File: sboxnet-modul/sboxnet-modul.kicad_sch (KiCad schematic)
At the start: 33 parts, among them J2 Conn_02x03_Odd_Even, J4 8P8C, J5 8P8C, J6 sboxnet-buchse_2x17, SW1 SW_Push, U1 MCP1703A-3302_SOT223, U2 MCP1703A-5002_SOT223, U3 SN65HVD230, U4 ATxmega128A4U-AU, Y1 16MHz

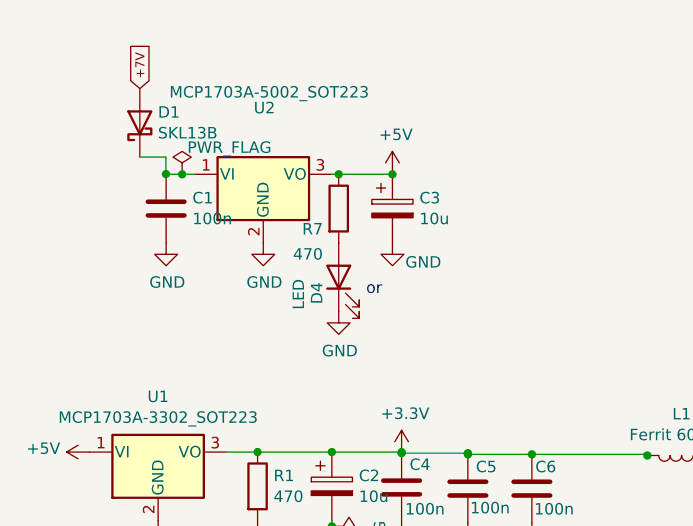
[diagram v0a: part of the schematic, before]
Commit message: sboxnet modul V6
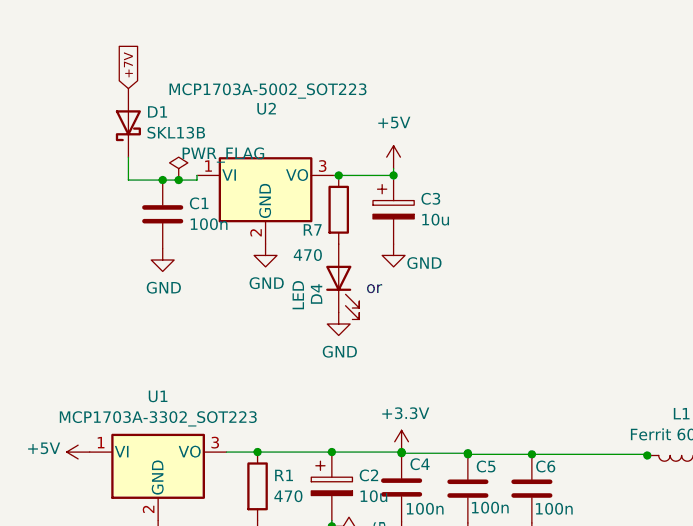
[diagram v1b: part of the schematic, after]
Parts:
- C3: footprint Capacitor_SMD:C_1206_3216Metric -> Capacitor_SMD:C_1206_3216Metric_Pad1.33x1.80mm_HandSolder
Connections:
- net at D1.1 (K): now also C1.2, U2.1 (VI)
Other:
- moved on the sheet: C1, D1
